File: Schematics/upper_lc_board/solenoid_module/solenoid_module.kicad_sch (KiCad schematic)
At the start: 9 parts, among them J1 SOL_CONN, U1 SSR_VO1400AEFTR

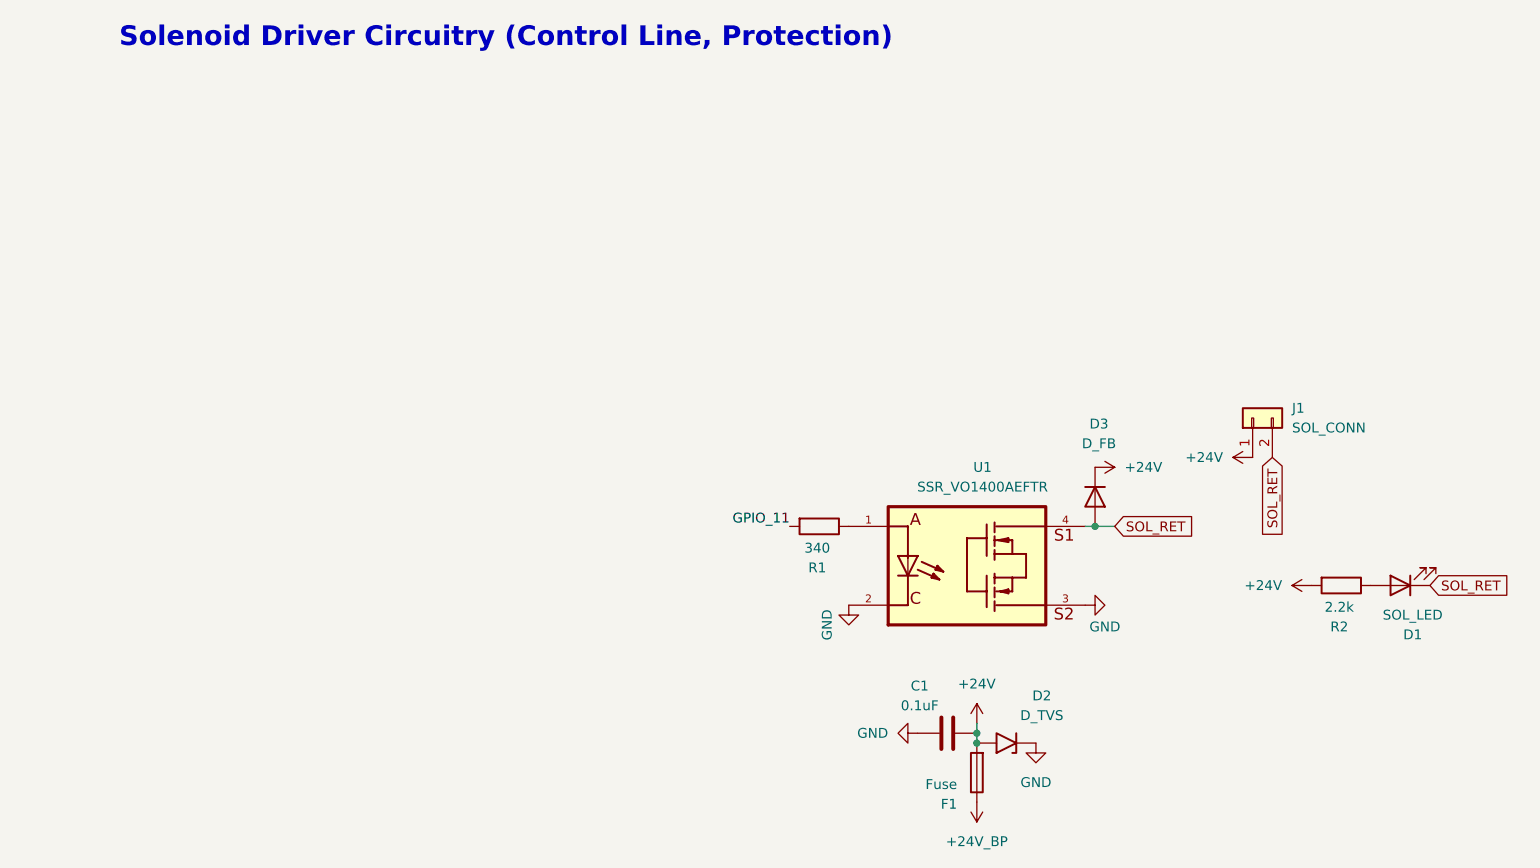
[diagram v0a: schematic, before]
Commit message: add hiearchical sheets in main board file
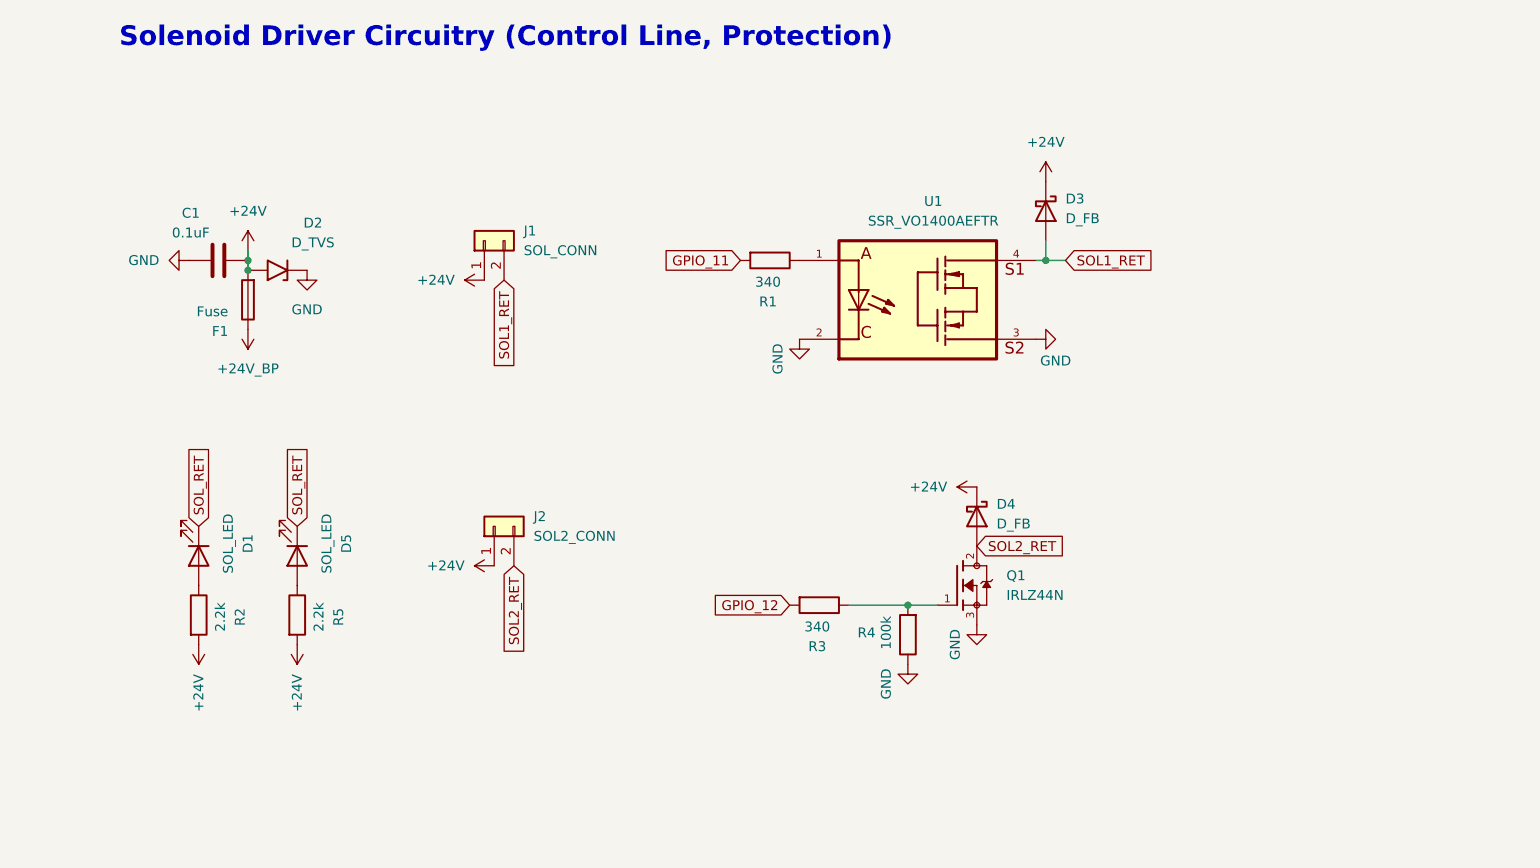
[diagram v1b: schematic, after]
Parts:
- removed D3: D_FB, symbol Device:D
- added D3, D4: D_FB, symbol Device:D_Schottky
- added D5: SOL_LED, symbol Device:LED
- added J2: SOL2_CONN, symbol Connector_Generic:Conn_01x02
- added Q1: IRLZ44N, IRLZ44N:TO254P1054X469X1930-3, symbol IRLZ44N:IRLZ44N
- added R3: 340, symbol Device:R
- added R4: 100k, symbol Device:R
- added R5: 2.2k, symbol Device:R
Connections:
- net +24V: now also D3.1 (K), D4.1 (K), J2.1 (Pin_1), R5.2
- net GND: now also Q1.3, R4.1
- net SOL_RET: now also D5.1 (K); no longer J1.2 (Pin_2), U1.4
- new net: D5.2 (A), R5.1
- new net: Q1.1, R3.1, R4.2
- new net GPIO_12: R3.2
- new net SOL1_RET: D3.2 (A), J1.2 (Pin_2), U1.4
- new net SOL2_RET: D4.2 (A), J2.2 (Pin_2), Q1.2
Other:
- moved on the sheet: C1, D1, D2, F1, J1, R1, R2, U1
